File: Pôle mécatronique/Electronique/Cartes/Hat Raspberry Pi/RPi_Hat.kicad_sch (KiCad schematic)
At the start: 9 parts, among them J1 Conn_02x03_Odd_Even, U1 XBee, U2 MCP25625-x-SS, Y1 8MHz

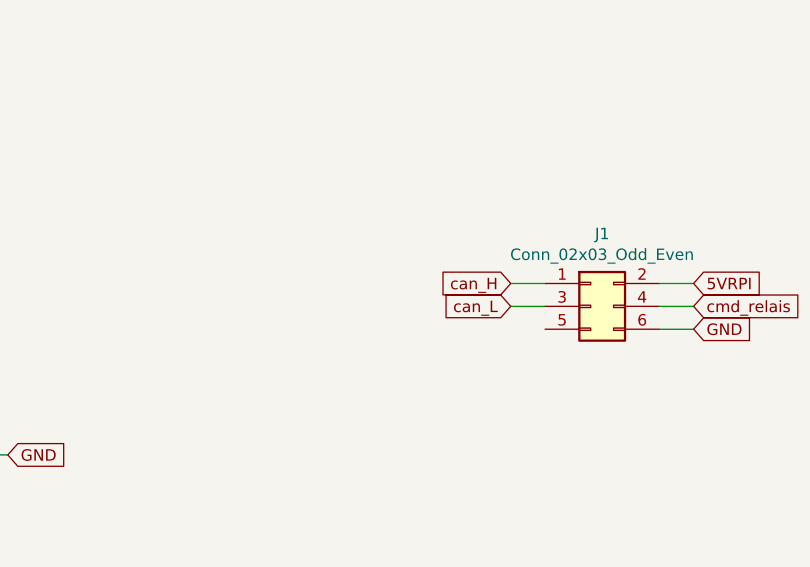
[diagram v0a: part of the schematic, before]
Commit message: Update alim correction
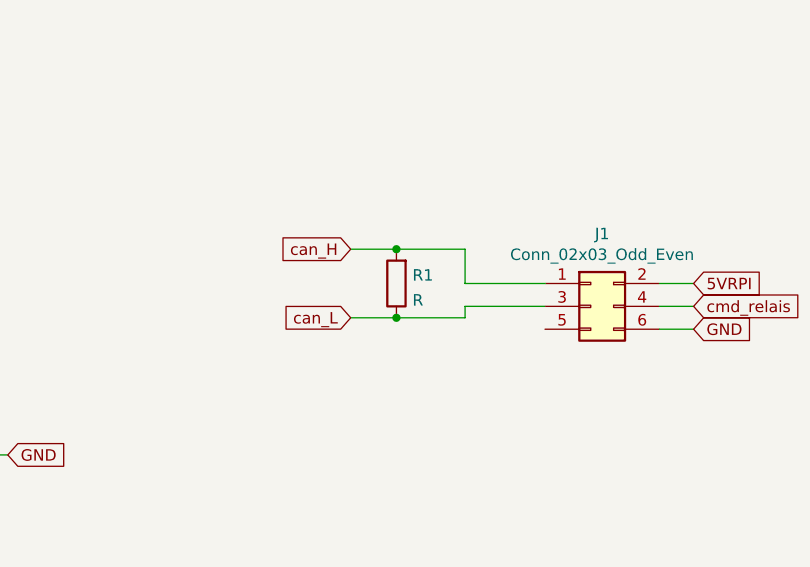
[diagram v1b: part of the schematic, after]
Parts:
- added R1: R, Resistor_THT:R_Axial_DIN0207_L6.3mm_D2.5mm_P2.54mm_Vertical, symbol Device:R
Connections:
- net can_H: now also R1.2
- net can_L: now also R1.1
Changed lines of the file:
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@@
   (junction (at 139.7 140.97) (diameter 0) (color 0 0 0 0)
   )
+  (junction (at 201.93 121.92) (diameter 0) (color 0 0 0 0)
+  )
   (junction (at 113.03 105.41) (diameter 0) (color 0 0 0 0)
   )
   (junction (at 118.11 167.64) (diameter 0) (color 0 0 0 0)
   )
+  (junction (at 201.93 129.54) (diameter 0) (color 0 0 0 0)
+  )
   (junction (at 156.21 144.78) (diameter 0) (color 0 0 0 0)
   )
@@
     (stroke (width 0) (type default) (color 0 0 0 0))
   )
+  (wire (pts (xy 201.93 121.92) (xy 209.55 121.92))
+    (stroke (width 0) (type default) (color 0 0 0 0))
+  )
   (wire (pts (xy 113.03 102.87) (xy 115.57 102.87))
     (stroke (width 0) (type default) (color 0 0 0 0))
@@
     (stroke (width 0) (type default) (color 0 0 0 0))
   )
+  (wire (pts (xy 196.85 129.54) (xy 201.93 129.54))
+    (stroke (width 0) (type default) (color 0 0 0 0))
+  )
   (wire (pts (xy 100.33 125.73) (xy 102.87 125.73))
     (stroke (width 0) (type default) (color 0 0 0 0))
@@
     (stroke (width 0) (type default) (color 0 0 0 0))
   )
+  (wire (pts (xy 196.85 121.92) (xy 201.93 121.92))
+    (stroke (width 0) (type default) (color 0 0 0 0))
+  )
   (wire (pts (xy 134.62 105.41) (xy 138.43 105.41))
     (stroke (width 0) (type default) (color 0 0 0 0))
@@
     (stroke (width 0) (type default) (color 0 0 0 0))
   )
+  (wire (pts (xy 209.55 128.27) (xy 209.55 129.54))
+    (stroke (width 0) (type default) (color 0 0 0 0))
+  )
   (wire (pts (xy 123.19 163.83) (xy 123.19 167.64))
     (stroke (width 0) (type default) (color 0 0 0 0))
@@
     (stroke (width 0) (type default) (color 0 0 0 0))
   )
+  (wire (pts (xy 209.55 125.73) (xy 218.44 125.73))
+    (stroke (width 0) (type default) (color 0 0 0 0))
+  )
   (wire (pts (xy 100.33 153.67) (xy 102.87 153.67))
     (stroke (width 0) (type default) (color 0 0 0 0))
@@
     (stroke (width 0) (type default) (color 0 0 0 0))
   )
-  (wire (pts (xy 214.63 128.27) (xy 218.44 128.27))
-    (stroke (width 0) (type default) (color 0 0 0 0))
-  )
   (wire (pts (xy 107.95 72.39) (xy 107.95 76.2))
     (stroke (width 0) (type default) (color 0 0 0 0))
@@
     (stroke (width 0) (type default) (color 0 0 0 0))
   )
+  (wire (pts (xy 218.44 128.27) (xy 209.55 128.27))
+    (stroke (width 0) (type default) (color 0 0 0 0))
+  )
   (wire (pts (xy 135.89 128.27) (xy 133.35 128.27))
     (stroke (width 0) (type default) (color 0 0 0 0))
   )
+  (wire (pts (xy 209.55 121.92) (xy 209.55 125.73))
+    (stroke (width 0) (type default) (color 0 0 0 0))
+  )
   (wire (pts (xy 128.27 48.26) (xy 134.62 48.26))
     (stroke (width 0) (type default) (color 0 0 0 0))
@@
     (stroke (width 0) (type default) (color 0 0 0 0))
   )
-  (wire (pts (xy 214.63 125.73) (xy 218.44 125.73))
-    (stroke (width 0) (type default) (color 0 0 0 0))
-  )
   (wire (pts (xy 123.19 105.41) (xy 127 105.41))
     (stroke (width 0) (type default) (color 0 0 0 0))
@@
   )
   (wire (pts (xy 139.7 140.97) (xy 148.59 140.97))
+    (stroke (width 0) (type default) (color 0 0 0 0))
+  )
+  (wire (pts (xy 201.93 129.54) (xy 209.55 129.54))
     (stroke (width 0) (type default) (color 0 0 0 0))
   )
@@
     )
   )
-  (global_label "can_L" (shape input) (at 214.63 128.27 180) (fields_autoplaced)
-    (effects (font (size 1.27 1.27)) (justify right))
-    (property "Intersheet References" "${INTERSHEET_REFS}" (id 0) (at 189.23 57.15 0)
+  (global_label "can_L" (shape input) (at 196.85 129.54 180) (fields_autoplaced)
+    (effects (font (size 1.27 1.27)) (justify right))
+    (property "Intersheet References" "${INTERSHEET_REFS}" (id 0) (at 171.45 58.42 0)
       (effects (font (size 1.27 1.27)) hide)
     )
@@
     )
   )
-  (global_label "can_H" (shape input) (at 214.63 125.73 180) (fields_autoplaced)
-    (effects (font (size 1.27 1.27)) (justify right))
-    (property "Intersheet References" "${INTERSHEET_REFS}" (id 0) (at 189.23 59.69 0)
+  (global_label "can_H" (shape input) (at 196.85 121.92 180) (fields_autoplaced)
+    (effects (font (size 1.27 1.27)) (justify right))
+    (property "Intersheet References" "${INTERSHEET_REFS}" (id 0) (at 171.45 55.88 0)
       (effects (font (size 1.27 1.27)) hide)
     )
@@
     )
     (property "Description" "1k-10k" (id 4) (at 93.98 133.35 90))
+    (pin "1")
+    (pin "2")
+  )
+  (symbol (lib_id "Device:R") (at 201.93 125.73 180) (unit 1)
+    (in_bom yes) (on_board yes) (fields_autoplaced)
+    (property "Reference" "R1" (id 0) (at 203.708 124.8215 0)
+      (effects (font (size 1.27 1.27)) (justify right))
+    )
+    (property "Value" "R" (id 1) (at 203.708 127.5966 0)
+      (effects (font (size 1.27 1.27)) (justify right))
+    )
+    (property "Footprint" "Resistor_THT:R_Axial_DIN0207_L6.3mm_D2.5mm_P2.54mm_Vertical" (id 2) (at 203.708 125.73 90)
+      (effects (font (size 1.27 1.27)) hide)
+    )
+    (property "Datasheet" "~" (id 3) (at 201.93 125.73 0)
+      (effects (font (size 1.27 1.27)) hide)
+    )
     (pin "1")
     (pin "2")
@@
       (reference "J2") (unit 1) (value "RPi_GPIO") (footprint "RPi_Hat:Pin_Header_Straight_2x20")
     )
+    (path "/5d503d09-3382-41b1-85dd-a984512b456d"
+      (reference "R1") (unit 1) (value "R") (footprint "Resistor_THT:R_Axial_DIN0207_L6.3mm_D2.5mm_P2.54mm_Vertical")
+    )
     (path "/47b96755-77b4-4d1f-b7c7-e83301b841d7"
